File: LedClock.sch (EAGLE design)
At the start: 36 parts

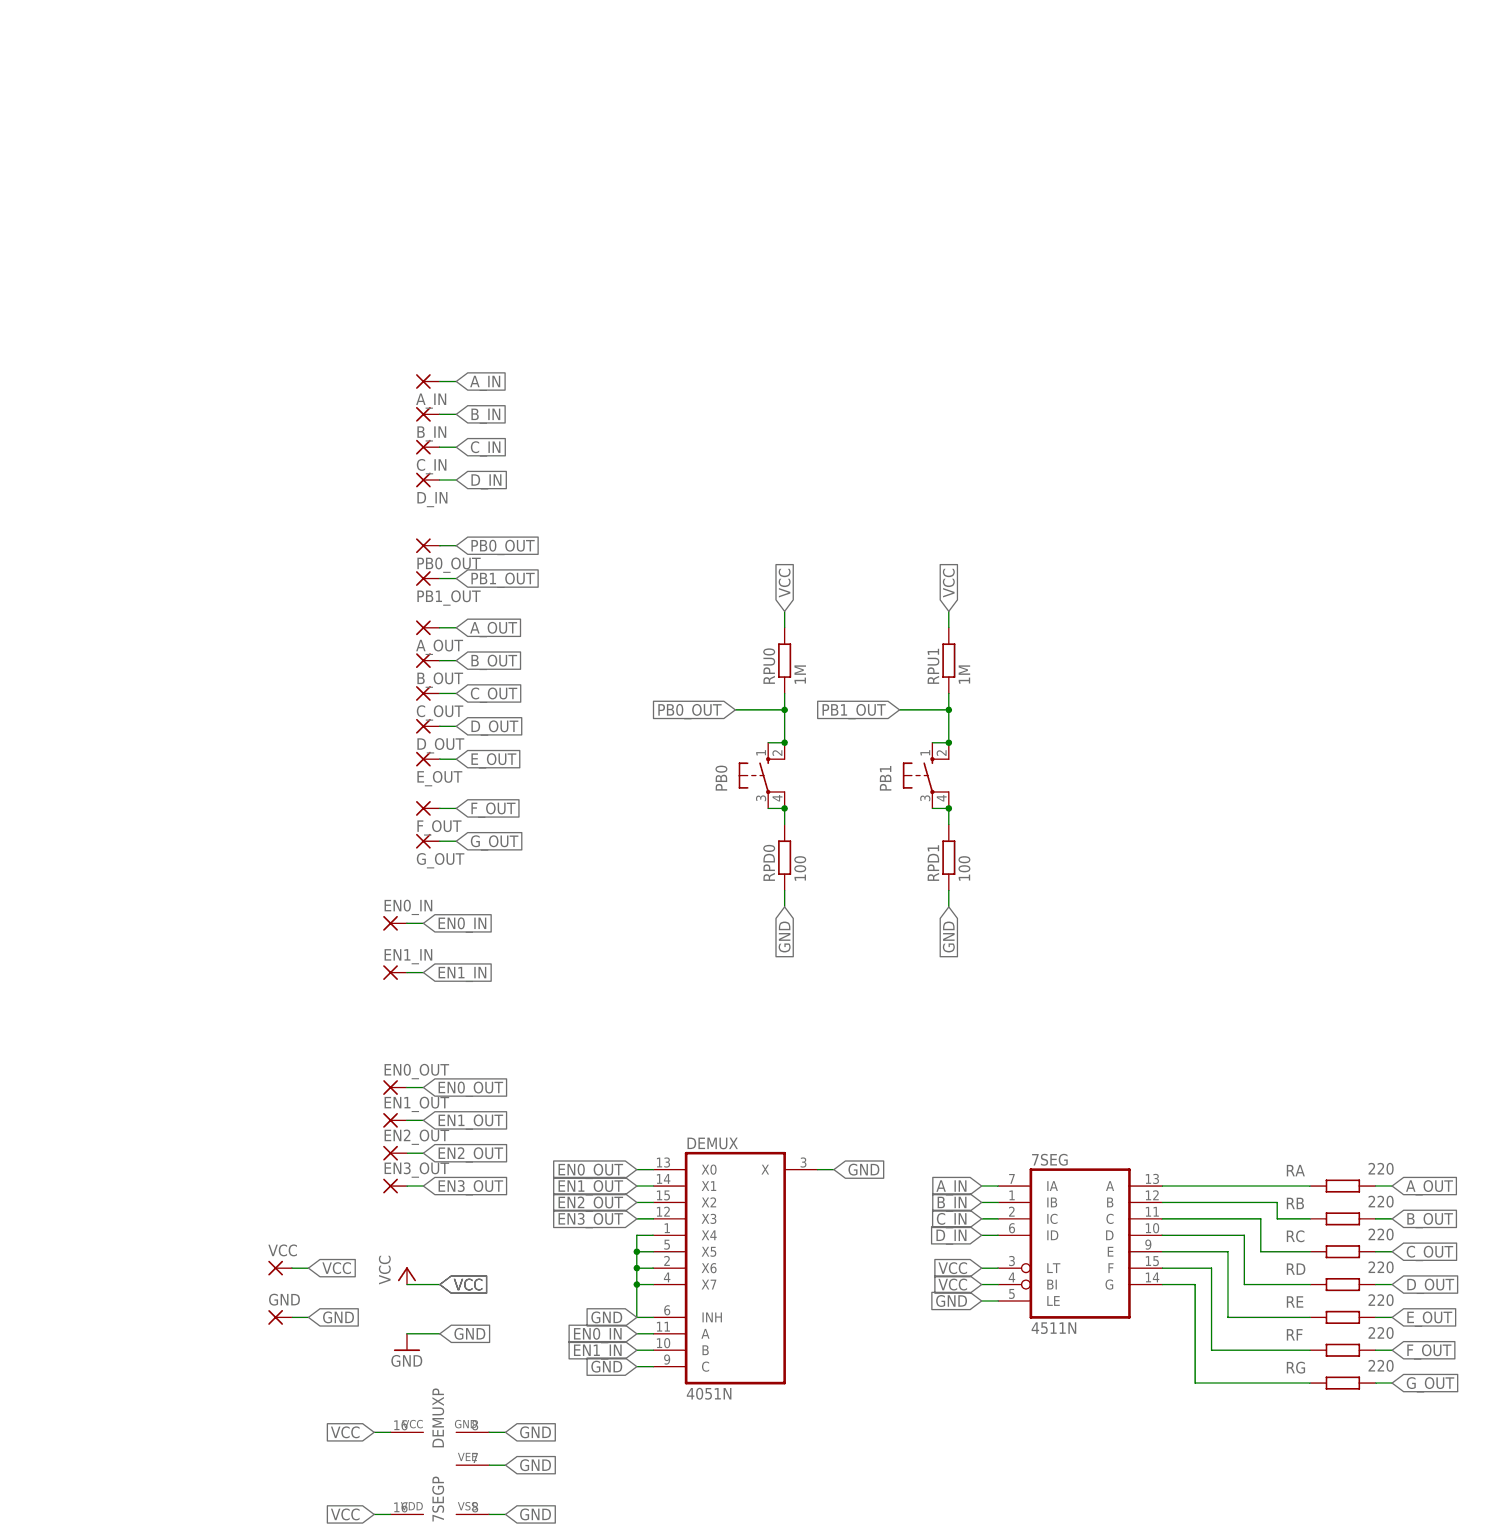
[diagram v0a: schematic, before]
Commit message: All parts are added. schematic_V0
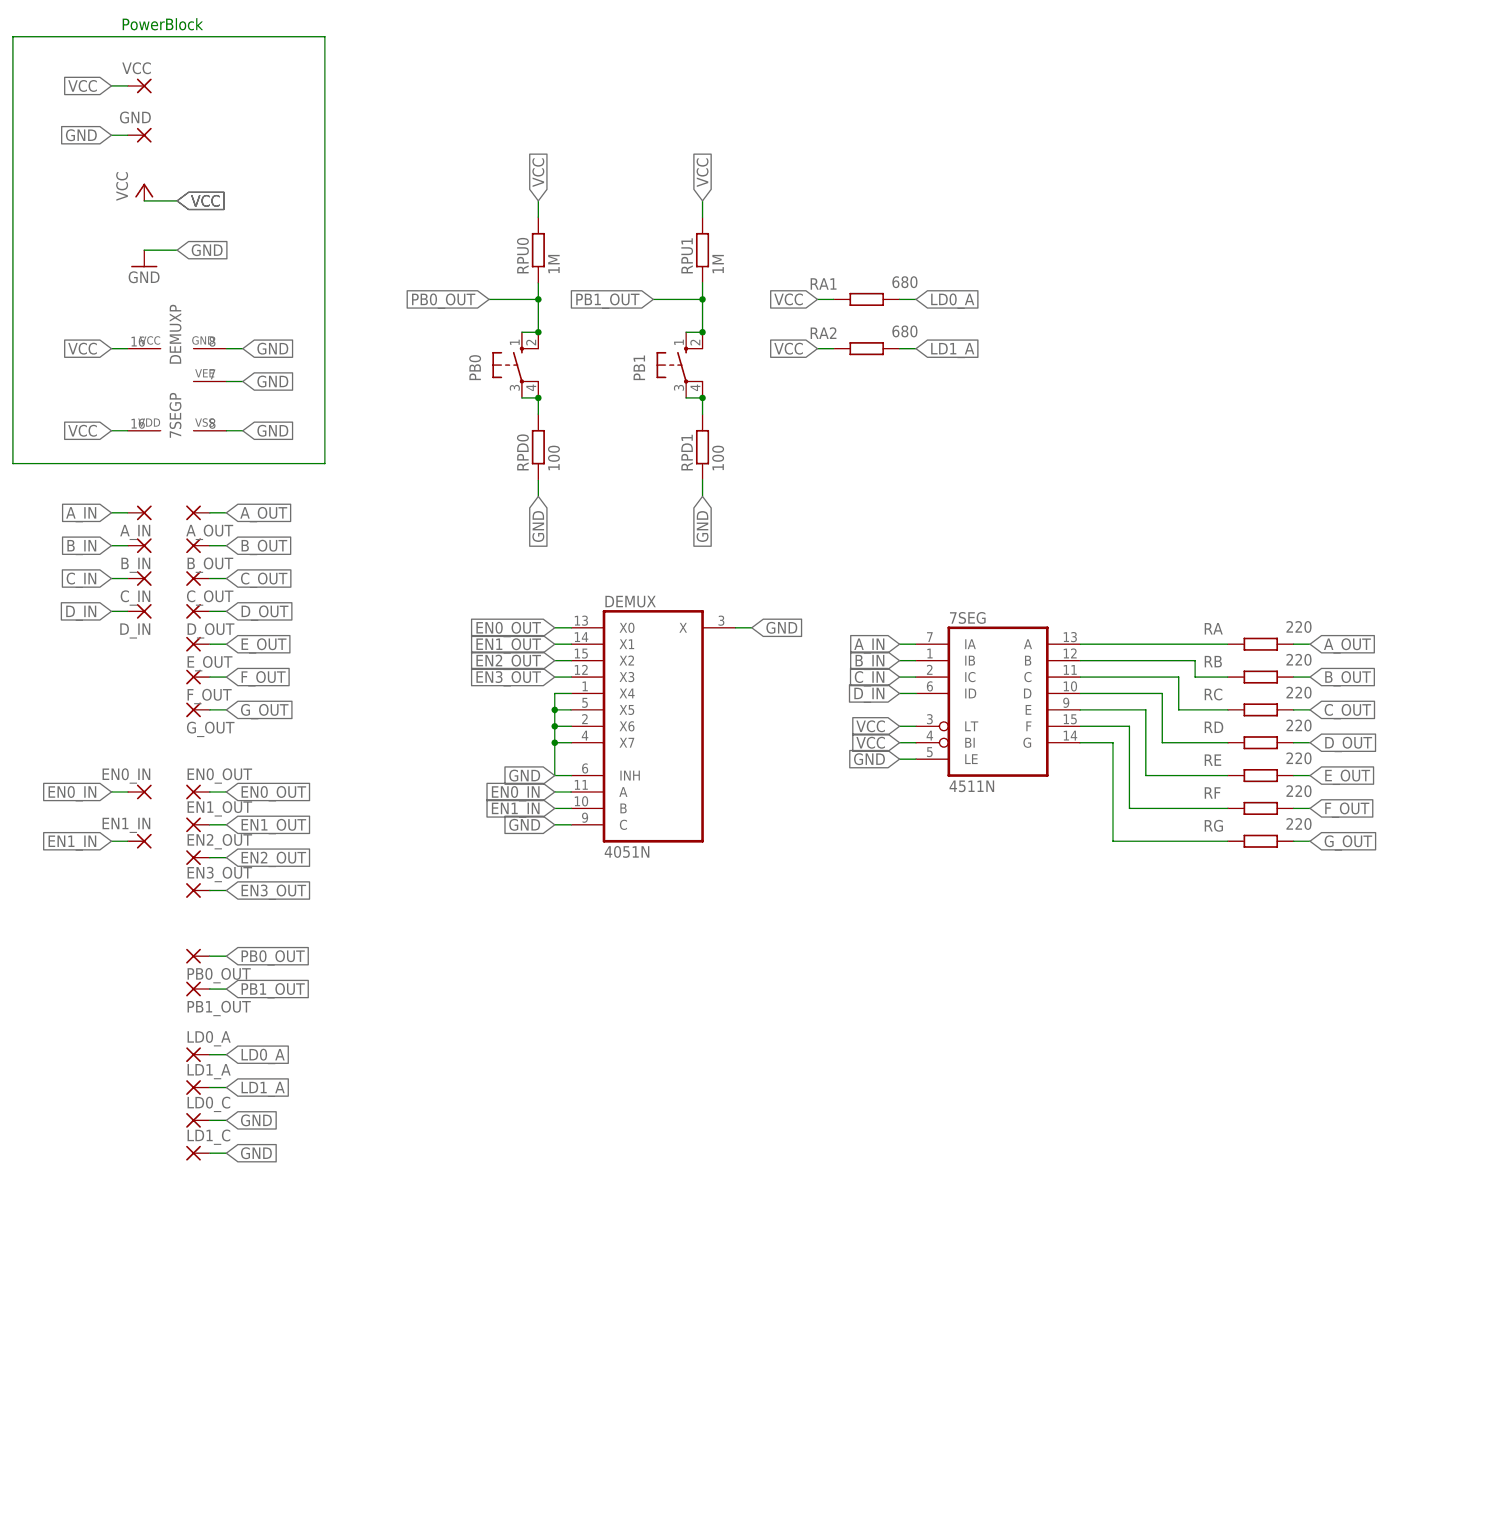
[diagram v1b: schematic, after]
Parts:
- added LD0_A, LD0_C, LD1_A, LD1_C: (no value), wirepad:2,54/1,0
- added RA1, RA2: 680, rcl:R-EU_R1206
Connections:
- new net LD0_A: LD0_A.P, RA1.2
- new net LD1_A: LD1_A.P, RA2.2
- net GND: now also LD0_C.P, LD1_C.P
- net VCC: now also RA1.1, RA2.1
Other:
- note added: "PowerBlock"
- moved on the sheet: 7SEG, 7SEGP, A_IN, A_OUT, B_IN, B_OUT, C_IN, C_OUT, DEMUX, DEMUXP, D_IN, D_OUT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
